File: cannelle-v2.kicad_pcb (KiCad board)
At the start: 2 copper layers, 62 parts, among them P1 USB_OTG, P2 CONN_02X04, P3 CONN_02X22, P4 CONN_02X22, SW1 SW_PUSH, U1 74LS157, U2 ATMEGA16U4-A, U3 SST25VF020B, U4 LD1117S12TR, U5 NCP1117ST33T3G, U6 ICE40HX1K-VQ100, X1 8MHz, X2 IQXO/7X

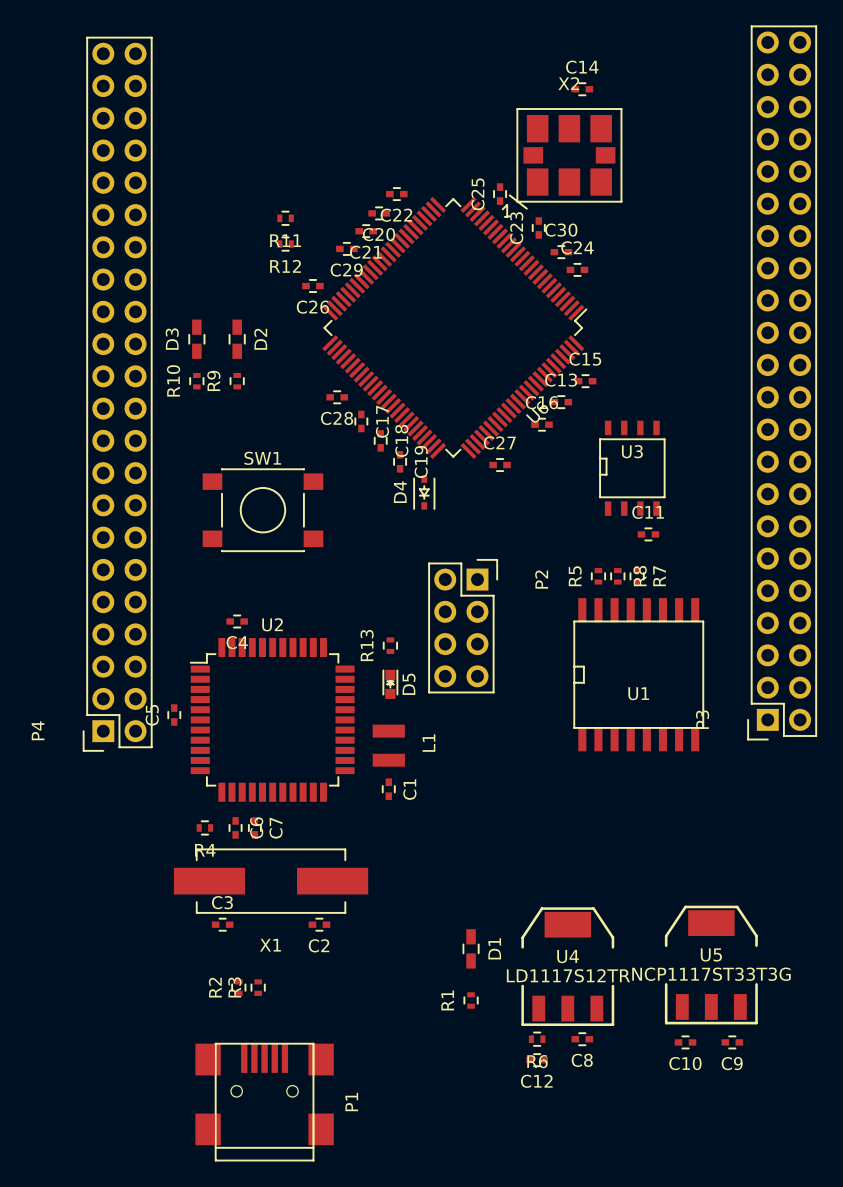
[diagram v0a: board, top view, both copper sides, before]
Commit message: Ordered labels
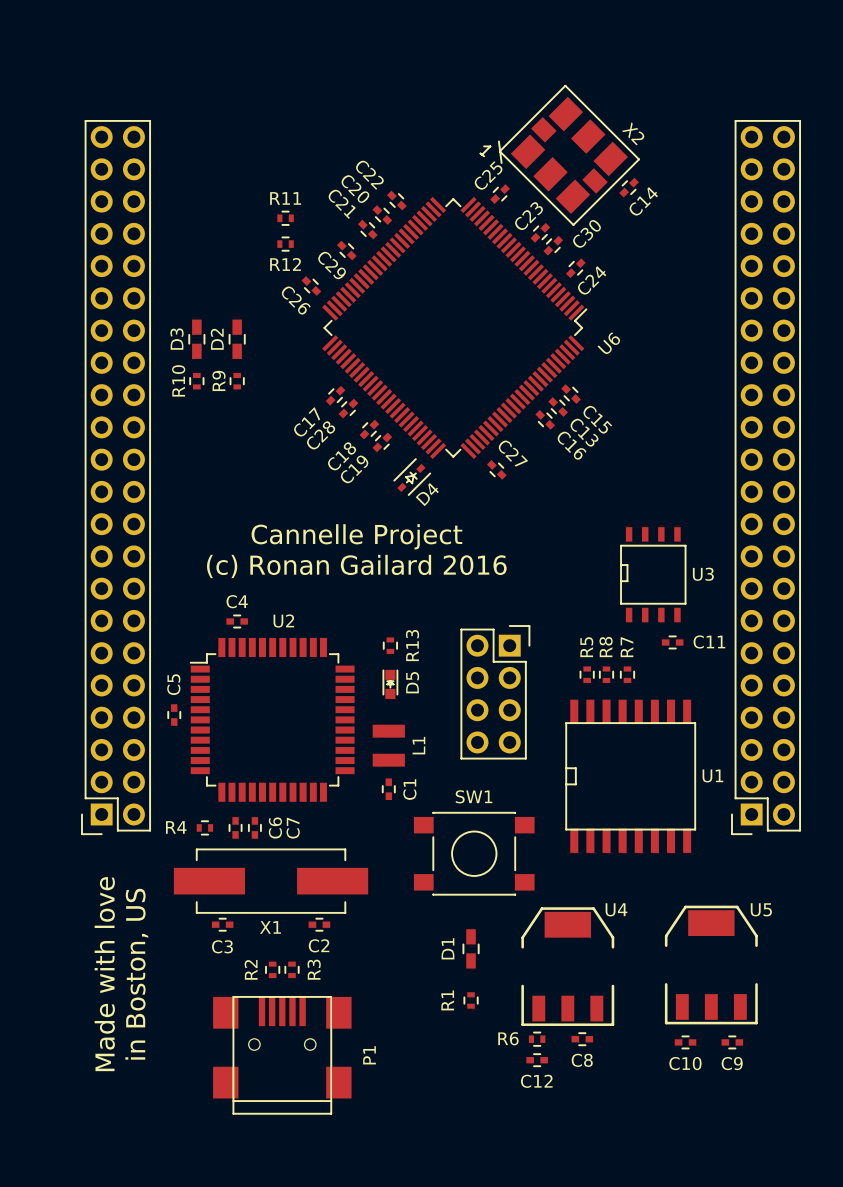
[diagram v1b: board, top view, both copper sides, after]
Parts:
- ?: renamed from P2; value CONN_02X04 -> (none)
- ?: renamed from P3; value CONN_02X22 -> (none)
- ?: renamed from P4; value CONN_02X22 -> (none)
- C1, C4, C5: value 1u -> (none)
- C10, C11, C12, C13, C14, C15, C16, C17, C18, C19, C20, C21, C22, C23, C24, C25, C26, C27, C28, C29, C30, C6, C7, C8, C9: value 100nF -> (none)
- C2, C3: value 22p -> (none)
- D1, D2, D3, D5: value LED -> (none)
- D4: value D_Schottky -> (none)
- R1: value 370 -> (none)
- R10, R12, R9: value 2.2k -> (none)
- R11, R4, R5, R7, R8: value 10k -> (none)
- R13, R2, R3: value 22 -> (none)
- R6: value 120 -> (none)
- SW1: value SW_PUSH -> (none)
- U1: value 74LS157 -> (none)
- U2: value ATMEGA16U4-A -> (none)
- U3: value SST25VF020B -> (none)
- U4: value LD1117S12TR -> (none)
- U5: value NCP1117ST33T3G -> (none)
- U6: value ICE40HX1K-VQ100 -> ICE40HX1K
- X1: value 8MHz -> (none)
- X2: value IQXO/7X -> (none)
- moved SW1 31.8 mm to (147.3, 101.1)
- moved C11 8.72 mm to (162.9, 84.5)
- moved C14 8.58 mm to (159.5, 48.6), turned to 45 degrees
- moved U3 8.54 mm to (161.4, 79.1)
- moved U1 8.03 mm to (159.6, 95.0)
- moved R5 7.80 mm to (156.2, 87.0)
- moved R8 7.80 mm to (157.7, 87.0)
- moved R7 7.78 mm to (159.4, 87.0)
- moved ? 7.56 mm to (169.2, 98.0)
- moved ? 6.56 mm to (118.0, 98.0)
- moved ? 5.79 mm to (150.1, 84.7)
- moved P1 3.94 mm to (132.2, 117.0)
- moved R2 3.01 mm to (131.4, 110.2)
- moved R3 3.01 mm to (133.0, 110.2)
- moved C17 2.87 mm to (136.4, 65.0), turned to 225 degrees
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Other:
- board text added: "Cannelle Project (c) Ronan Gailard 2016"
- board text added: "Made with love in Boston, US"
